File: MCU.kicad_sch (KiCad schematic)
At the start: 35 parts, among them SW1 RESET, SW2 USR_SW_1, SW3 USR_SW_2, SW4 SW_DIP_x04, U1 STM32h553VITx, Y1 Crystal

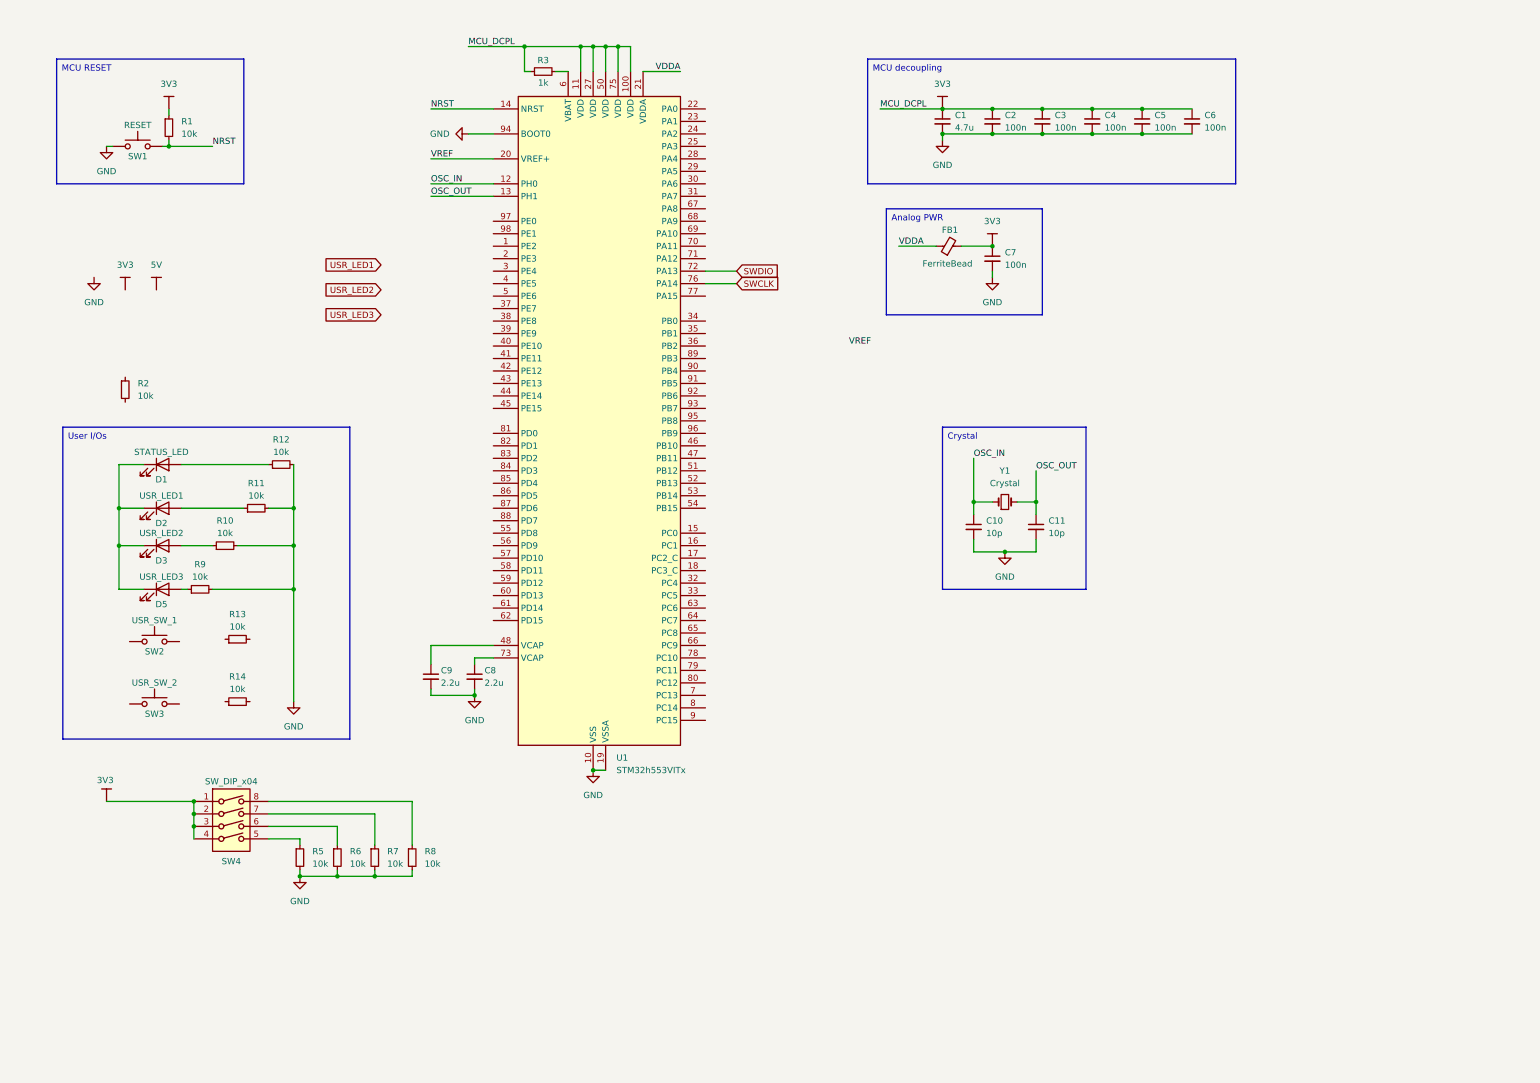
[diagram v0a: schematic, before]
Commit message: Various updates
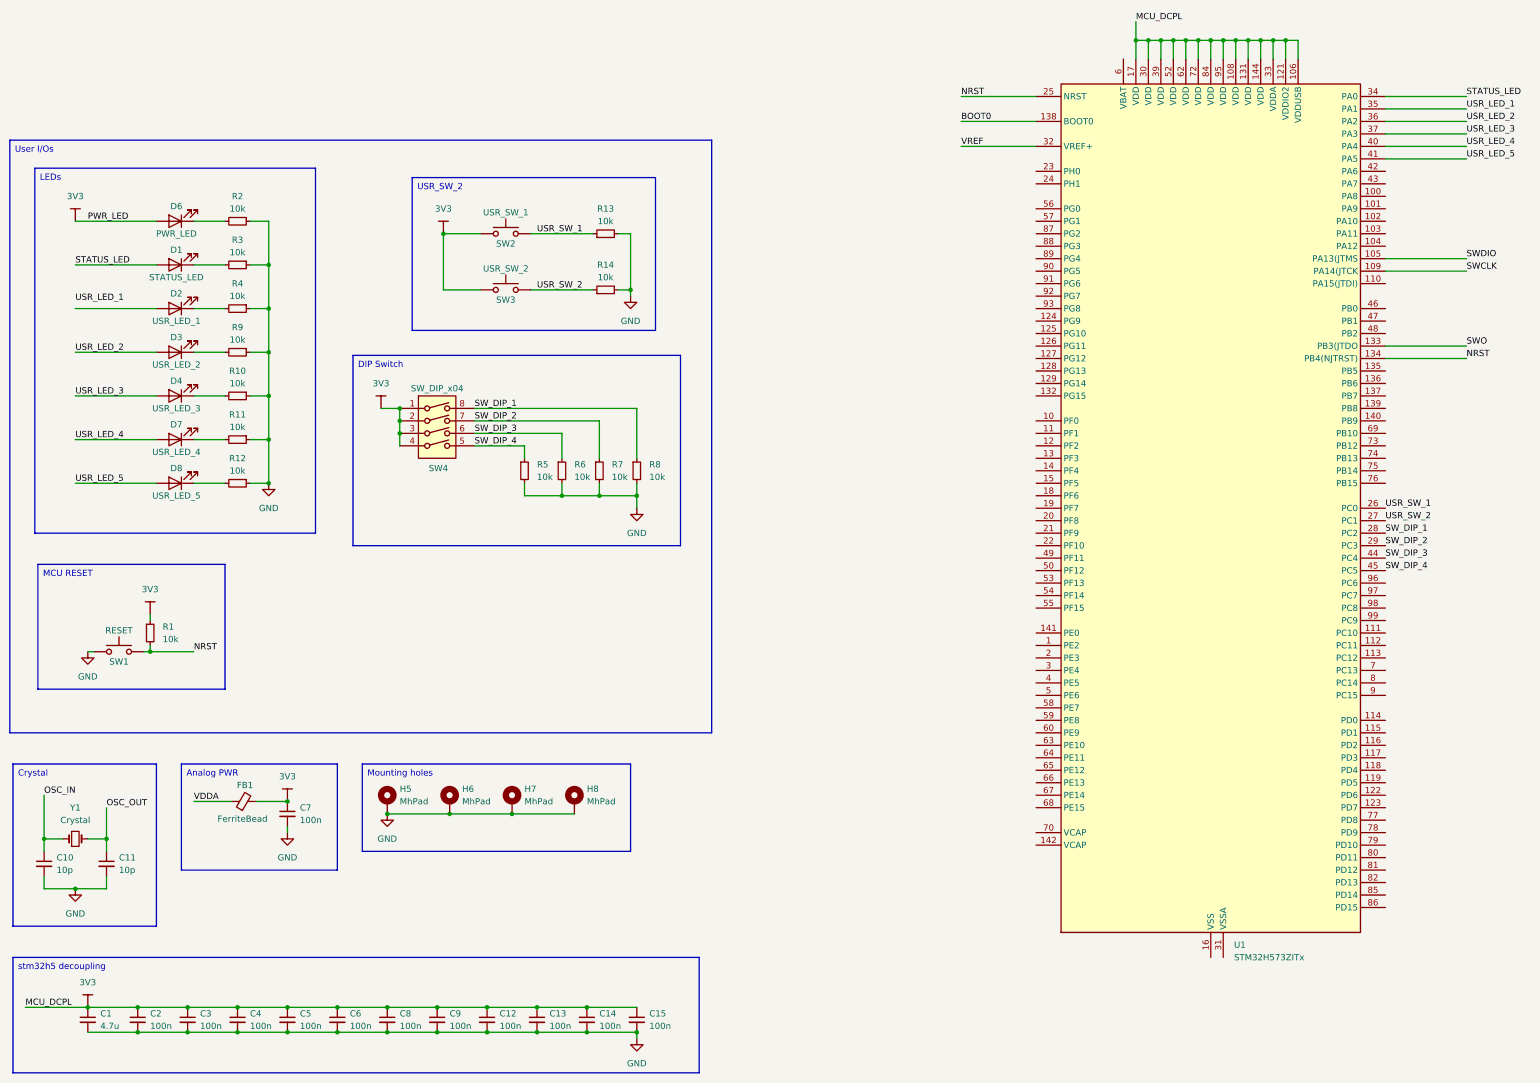
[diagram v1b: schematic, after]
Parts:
- removed D5: USR_LED3, symbol Device:LED
- removed R3: 1k, symbol MyLib:R
- removed U1: STM32h553VITx, Package_QFP:LQFP-100_14x14mm_P0.5mm, symbol MCU_ST_STM32h5:STM32h553VITx
- added C12, C13, C14, C15: 100n, symbol Device:C_Small
- added D4: USR_LED_3, symbol Device:LED
- added D6: PWR_LED, symbol Device:LED
- added D7: USR_LED_4, symbol Device:LED
- added D8: USR_LED_5, symbol Device:LED
- added H5, H6, H7, H8: MhPad, symbol MyLib:MhPad
- added R3, R4: 10k, symbol Device:R_Small
- added U1: STM32H573ZITx, Package_QFP:LQFP-144_20x20mm_P0.5mm, symbol MCU_ST_STM32H5:STM32H573ZITx
- C8, C9: value 2.2u -> 100n
- D2: value USR_LED1 -> USR_LED_1
- D3: value USR_LED2 -> USR_LED_2
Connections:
- net 3V3: now also C8.1, C9.1, SW2.1, SW3.1, C12.1, C13.1, C14.1, C15.1, D6.2 (A), U1.106 (VDDUSB), U1.108 (VDD), U1.121 (VDDIO2), U1.131 (VDD), U1.144 (VDD), U1.17 (VDD), U1.30 (VDD), U1.33 (VDDA), U1.39 (VDD), U1.52 (VDD), U1.62 (VDD), U1.72 (VDD), U1.84 (VDD), U1.95 (VDD)
- net GND: now also R10.1, R11.1, R12.1, R13.2, R14.2, R2.1, R9.1, C12.2, C13.2, C14.2, C15.2, H5.1, H6.1, H7.1, H8.1, R3.1, R4.1; no longer R10.2, R11.2, R12.2, R9.2
- net NRST: now also U1.134 (PB4(NJTRST)), U1.25 (NRST)
- net SWCLK: now also U1.109 (PA14(JTCK)
- net SWDIO: now also U1.105 (PA13(JTMS)
- net VREF: now also U1.32 (VREF+)
- net STATUS_LED: now reaches D1.2 (A)
- net STATUS_LED: now also U1.34 (PA0); no longer R12.1
- net SW_DIP_1: now reaches R8.1, SW4.8
- net SW_DIP_1: now also U1.28 (PC2)
- net USR_SW_2: now reaches SW3.2
- net USR_SW_2: now also R14.1, U1.27 (PC1)
- net USR_SW_1: now reaches SW2.2
- net USR_SW_1: now also R13.1, U1.26 (PC0)
- net SW_DIP_4: now reaches R5.1, SW4.5
- net SW_DIP_4: now also U1.45 (PC5)
- net at R2.2: now also D6.1 (K)
- net USR_LED_2: now reaches D3.2 (A)
- net USR_LED_2: now also U1.36 (PA2); no longer R10.1
- net SW_DIP_3: now reaches R6.1, SW4.6
- net SW_DIP_3: now also U1.44 (PC4)
- net SW_DIP_2: now reaches R7.1, SW4.7
- net SW_DIP_2: now also U1.29 (PC3)
- net at D2.2 (A): no longer R11.1
- new net: D1.1 (K), R3.2
- new net: D7.1 (K), R11.2
- new net: D4.1 (K), R10.2
- new net: D3.1 (K), R9.2
- new net: D2.1 (K), R4.2
- new net: D8.1 (K), R12.2
- new net: U1.107 (VSS), U1.120 (VSS), U1.130 (VSS), U1.143 (VSS), U1.16 (VSS), U1.38 (VSS), U1.51 (VSS), U1.61 (VSS), U1.71 (VSS), U1.83 (VSS), U1.94 (VSS)
- new net BOOT0: U1.138 (BOOT0)
- new net SWO: U1.133 (PB3(JTDO)
- new net USR_LED_1: U1.35 (PA1)
- new net USR_LED_3: D4.2 (A), U1.37 (PA3)
- new net USR_LED_4: D7.2 (A), U1.40 (PA4)
- new net USR_LED_5: D8.2 (A), U1.41 (PA5)
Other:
- moved on the sheet: C1, C10, C11, C2, C3, C4, C5, C7, D1, D2, D3, FB1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
